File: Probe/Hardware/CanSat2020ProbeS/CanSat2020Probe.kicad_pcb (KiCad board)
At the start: 2 copper layers, 56 x 56 mm, 35 parts, among them IC1 TESEO-LIV3F, J1 BME280, J2 MPU-9250, J3 Micro_SD_Card, J4 Conn_01x03_Male, J5 Conn_Coaxial, J6 Conn_Coaxial, J7 Conn_01x05_Male, J8 Conn_01x02_Male, SW1 SW_DIP_x01, U1 STM32F411RETx, U2 RFM69W, U3 LD3985M33R_SOT23, Y1 Crystal

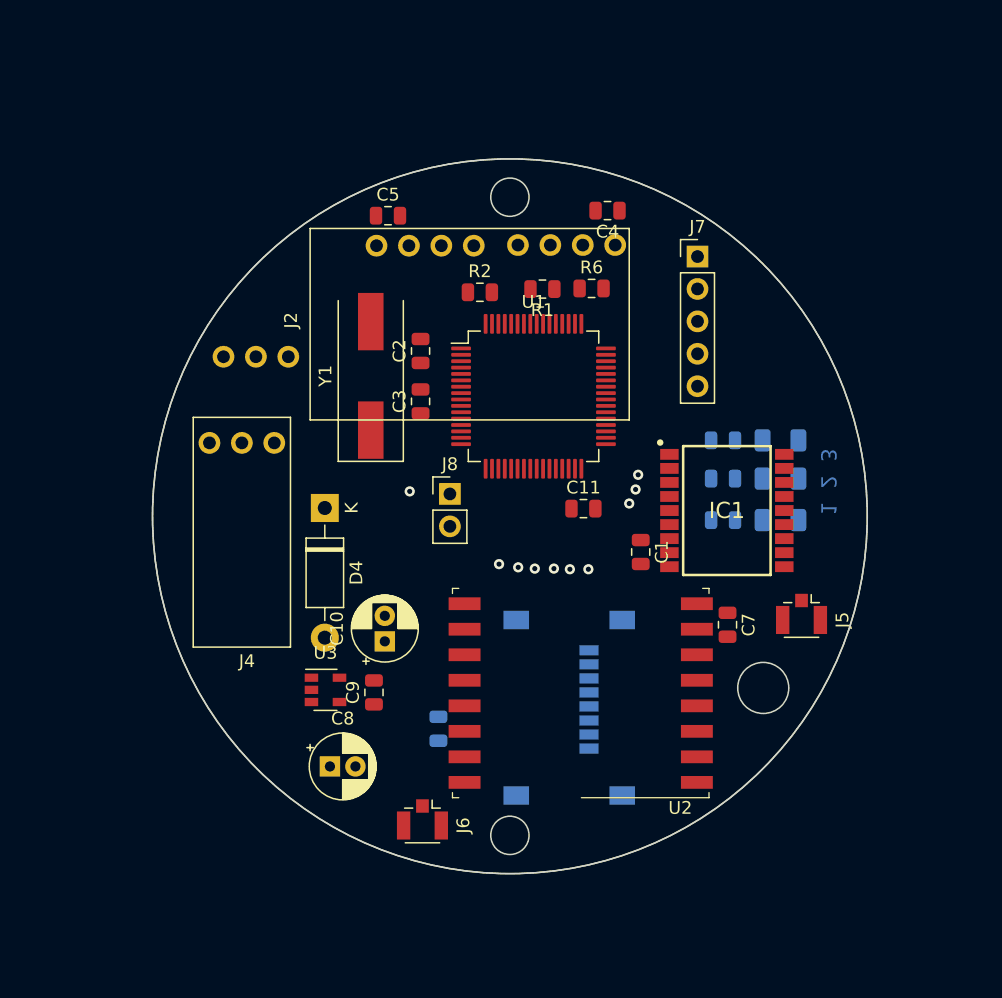
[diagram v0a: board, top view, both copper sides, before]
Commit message: minor improvements
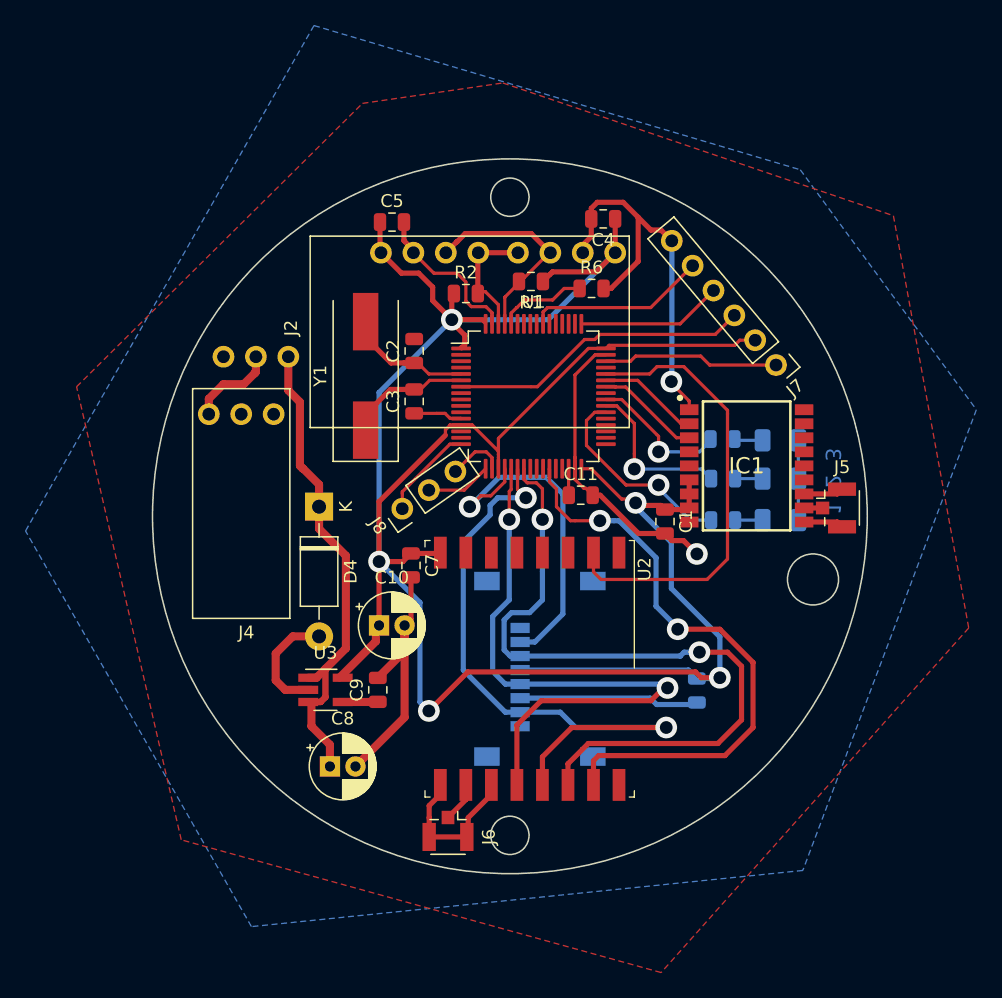
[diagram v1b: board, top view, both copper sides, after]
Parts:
- J7: value Conn_01x05_Male -> Conn_01x06_Male; footprint Connector_PinHeader_2.54mm:PinHeader_1x05_P2.54mm_Vertical -> Connector_PinHeader_2.54mm:PinHeader_1x06_P2.54mm_Vertical
- J8: value Conn_01x02_Male -> Conn_01x03_Male; footprint Connector_PinHeader_2.54mm:PinHeader_1x02_P2.54mm_Vertical -> Connector_PinHeader_2.54mm:PinHeader_1x03_P2.54mm_Vertical
- U3: footprint Package_TO_SOT_SMD:SOT-23-5 -> Package_TO_SOT_SMD:SOT-23-5_HandSoldering
- moved C7 25.2 mm to (142.2, 103.8)
- moved C6 20.5 mm to (164.7, 113.7)
- moved J7 10.5 mm to (170.8, 88.2), turned to 220 degrees
- moved J5 8.73 mm to (175.6, 99.3), turned to 0 degrees
- moved U2 4.43 mm to (151.6, 112.0), turned to 270 degrees
- moved J8 3.91 mm to (141.6, 99.4), turned to 125 degrees
- moved IC1 3.83 mm to (168.6, 96.0)
- moved J3 3.82 mm to (152.3, 112.0), turned to 270 degrees
- moved C1 3.05 mm to (162.2, 100.4)
- moved J4 2.25 mm to (128.9, 92.0)
- moved J6 2.19 mm to (145.2, 124.7)
- moved C10 1.33 mm to (139.8, 108.5), turned to 0 degrees
- moved R2 1.10 mm to (146.6, 82.5)
- moved R1 1.08 mm to (151.7, 81.6)
- moved C11 1.07 mm to (155.6, 98.3)
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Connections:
- J7 pad 1: /SWCLOCK -> /SWDIO
- J7 pad 2: /SWDIO -> +3V3
- J7 pad 3: /SWO -> /RST
- J7 pad 4: /RST -> /SWCLOCK
- J7 pad 5: GND -> /SWO
- U1 pad 27: Net-(U1-Pad27) -> /CS_RAD
- U1 pad 41: /CS_RAD -> Net-(U1-Pad41)
- U1 pad 46: Net-(U1-Pad46) -> /SWDIO
- U1 pad 50: /SWDIO -> Net-(U1-Pad50)
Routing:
- net +3V3: track 0.00 -> 204.4 mm, vias 1 -> 5
- net GND: track 0.00 -> 144.8 mm, vias 0 -> 2
- net /MOSI: track 0.00 -> 58.5 mm, vias 0 -> 2
- net /MISO: track 0.00 -> 50.4 mm, vias 0 -> 2
- net /SCK: track 0.00 -> 47.8 mm, vias 0 -> 2
- net /CS_RAD: track 0.00 -> 47.2 mm, vias 0 -> 2
- net +BATT: track 0.00 -> 38.1 mm
- net /DIO0: track 0.00 -> 36.5 mm
- net /CS_SD: track 0.00 -> 27.7 mm, vias 0 -> 1
- net /RST: track 0.00 -> 23.7 mm
- net /SCL: track 0.00 -> 17.2 mm
- net Net-(R3-Pad1): track 0.00 -> 15.9 mm, vias 0 -> 1
- net /SWO: track 0.00 -> 14.1 mm
- net /SWDIO: track 0.00 -> 13.8 mm
- net Net-(R4-Pad1): track 0.00 -> 12.2 mm, vias 0 -> 1
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- added copper zone on B.Cu, net GND
- added copper zone on F.Cu, net GND
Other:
- outline, holes or cut-outs redrawn
